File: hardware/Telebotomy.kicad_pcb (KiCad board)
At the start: 2 copper layers, 88 x 20.7 mm, 23 parts, among them J1 10118193-0001LF, J2 RJHSE-5080, J3 Conn_02x03_Odd_Even, J4 Conn_02x03_Odd_Even, J5 RJHSE-5080, J6 Conn_01x06_Pin, J7 Conn_01x04_Pin, U1 KSZ8863MLL, U2 ATTINY85-20PU, U3 MIC5504-3.3YM5_TR

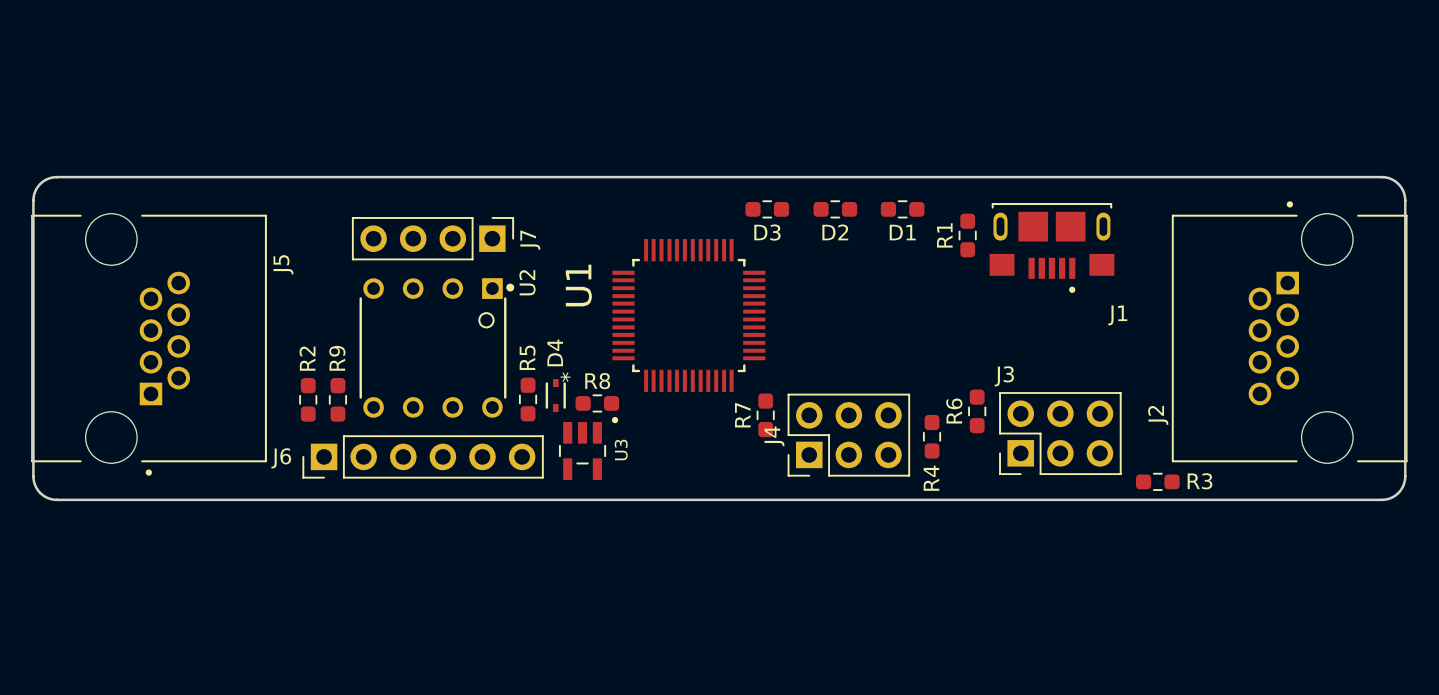
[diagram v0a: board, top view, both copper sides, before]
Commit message: PCB Updates
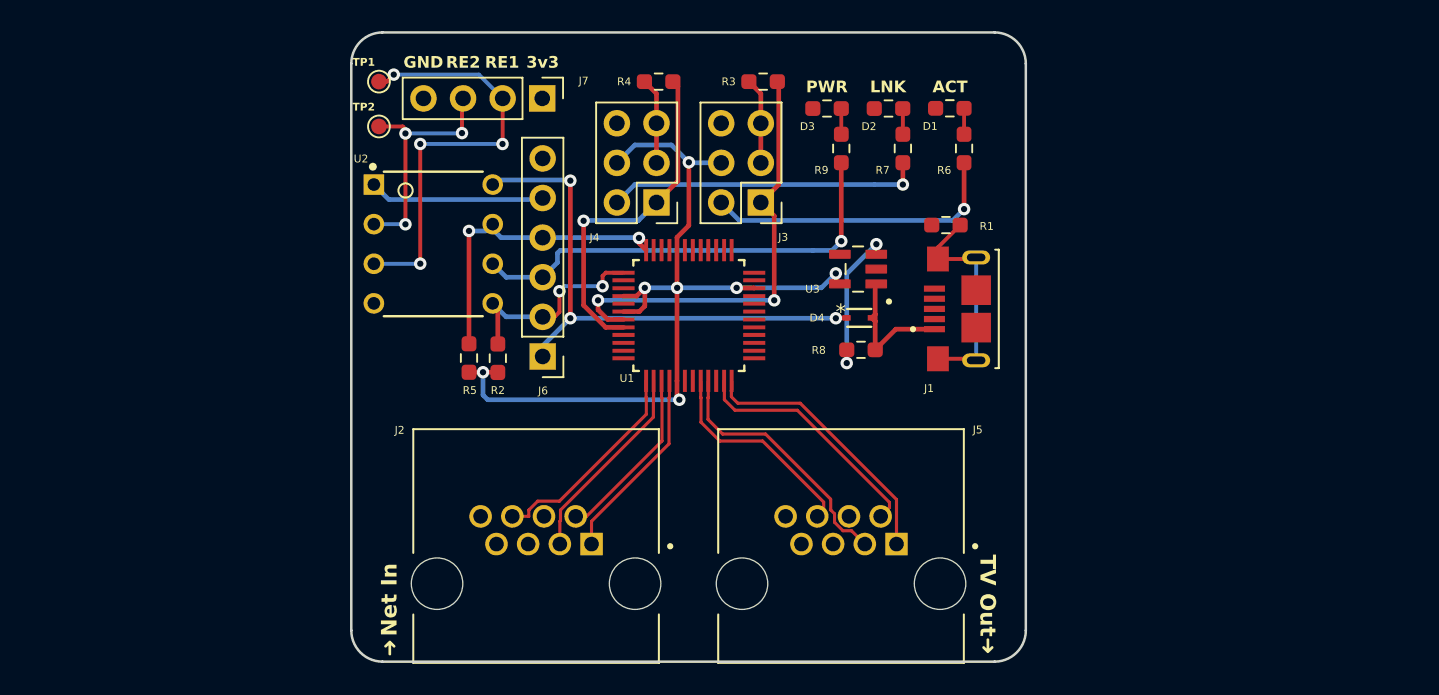
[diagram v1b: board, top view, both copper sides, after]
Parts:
- added G***: LOGO, telebotomy:arrow, F.Cu at (128.0, 114.5)
- added G***: LOGO, telebotomy:arrow, F.Cu at (166.4, 114.3)
- added G***: LOGO, telebotomy:lamemakes_logo, B.Cu at (162.1, 78.9)
- added TP1: TestPoint, TestPoint:TestPoint_Pad_D1.0mm, F.Cu at (127.3, 78.2)
- added TP2: TestPoint, TestPoint:TestPoint_Pad_D1.0mm, F.Cu at (127.3, 81.0)
- moved J2 53.1 mm to (137.4, 110.4), turned to 0 degrees
- moved J5 49.4 mm to (157.0, 110.4), turned to 0 degrees
- moved R9 36.1 mm to (157.0, 82.5)
- moved R3 36.0 mm to (152.0, 78.2), turned to 0 degrees
- moved R4 28.7 mm to (145.3, 78.2), turned to 0 degrees
- moved J3 23.2 mm to (151.8, 85.9), turned to 180 degrees
- moved U3 21.2 mm to (158.1, 90.2), turned to 180 degrees
- moved D4 20.1 mm to (158.1, 93.3), turned to 0 degrees
- moved R7 19.2 mm to (160.9, 82.5), turned to -90 degrees
- moved J4 18.9 mm to (145.1, 85.9), turned to 180 degrees
- moved R8 17.3 mm to (158.3, 95.4)
- moved R6 16.9 mm to (164.9, 82.5), turned to -90 degrees
- moved J6 15.4 mm to (137.8, 95.8), turned to 180 degrees
- moved R2 12.4 mm to (135.0, 95.9)
- moved J7 9.55 mm to (137.8, 79.2)
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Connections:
- J2 pad 1: /TXP2 -> /TX1_P
- J2 pad 2: /TXM2 -> /TX1_N
- J2 pad 3: /RXP2 -> /RX1_P
- J2 pad 6: /RXM2 -> /RX1_N
- J5 pad 1: /TXP1 -> /TX2_P
- J5 pad 2: /TXM1 -> /TX2_N
- J5 pad 3: /RXP1 -> /RX2_P
- J5 pad 6: /RXM1 -> /RX2_N
- U1 pad 1: /RXM1 -> /RX1_N
- U1 pad 11: /TXM1 -> /TX2_N
- U1 pad 12: /TXP2 -> /TX2_P
- U1 pad 2: /RXP1 -> /RX1_P
- U1 pad 3: /TXM1 -> /TX1_N
- U1 pad 4: /TXP1 -> /TX1_P
- U1 pad 8: /RXM2 -> /RX2_N
- U1 pad 9: /RXP1 -> /RX2_P
- U2 pad 2: /REM_IN1 -> /REM_IN2
- U2 pad 3: /REM_IN2 -> /REM_IN1
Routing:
- net /+3v3: track 0.00 -> 58.1 mm, vias 0 -> 7
- net /AT_PWR: track 0.00 -> 34.9 mm, vias 0 -> 3
- net /AT_LED: track 0.00 -> 29.1 mm, vias 0 -> 1
- net /P1LED1: track 0.00 -> 28.8 mm, vias 0 -> 2
- net /REM_IN1: track 0.00 -> 27.6 mm, vias 0 -> 4
- net /P1LED0: track 0.00 -> 22.2 mm, vias 0 -> 1
- net /LINK_LED: track 0.00 -> 20.2 mm, vias 0 -> 1
- net /SCL: track 0.00 -> 19.9 mm, vias 0 -> 2
- net /ACT_LED: track 0.00 -> 19.3 mm, vias 0 -> 1
- net /TX2_P: track 0.00 -> 17.2 mm
- net /RX2_P: track 0.00 -> 16.6 mm
- net /REM_IN2: track 0.00 -> 15.8 mm, vias 0 -> 3
- net /TX2_N: track 0.00 -> 15.7 mm
- net Net-(J1-SHIELD-PadS1): track 0.00 -> 14.3 mm
- net /SDA: track 0.00 -> 13.8 mm, vias 0 -> 2
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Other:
- board size 88 x 20.7 mm -> 43.3 x 40.4 mm
- board text added: "3v3"
- board text added: "ACT"
- board text added: "GND"
- board text added: "LNK"
- board text added: "Net In"
- board text added: "PWR"
- board text added: "RE1"
- board text added: "RE2"
- board text added: "TV Out"
